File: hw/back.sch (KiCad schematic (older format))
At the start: 26 parts, among them J1 IDC_02X13, U1 OSRB38C9BA, U2 MCP1826S, U3 MCP1826S

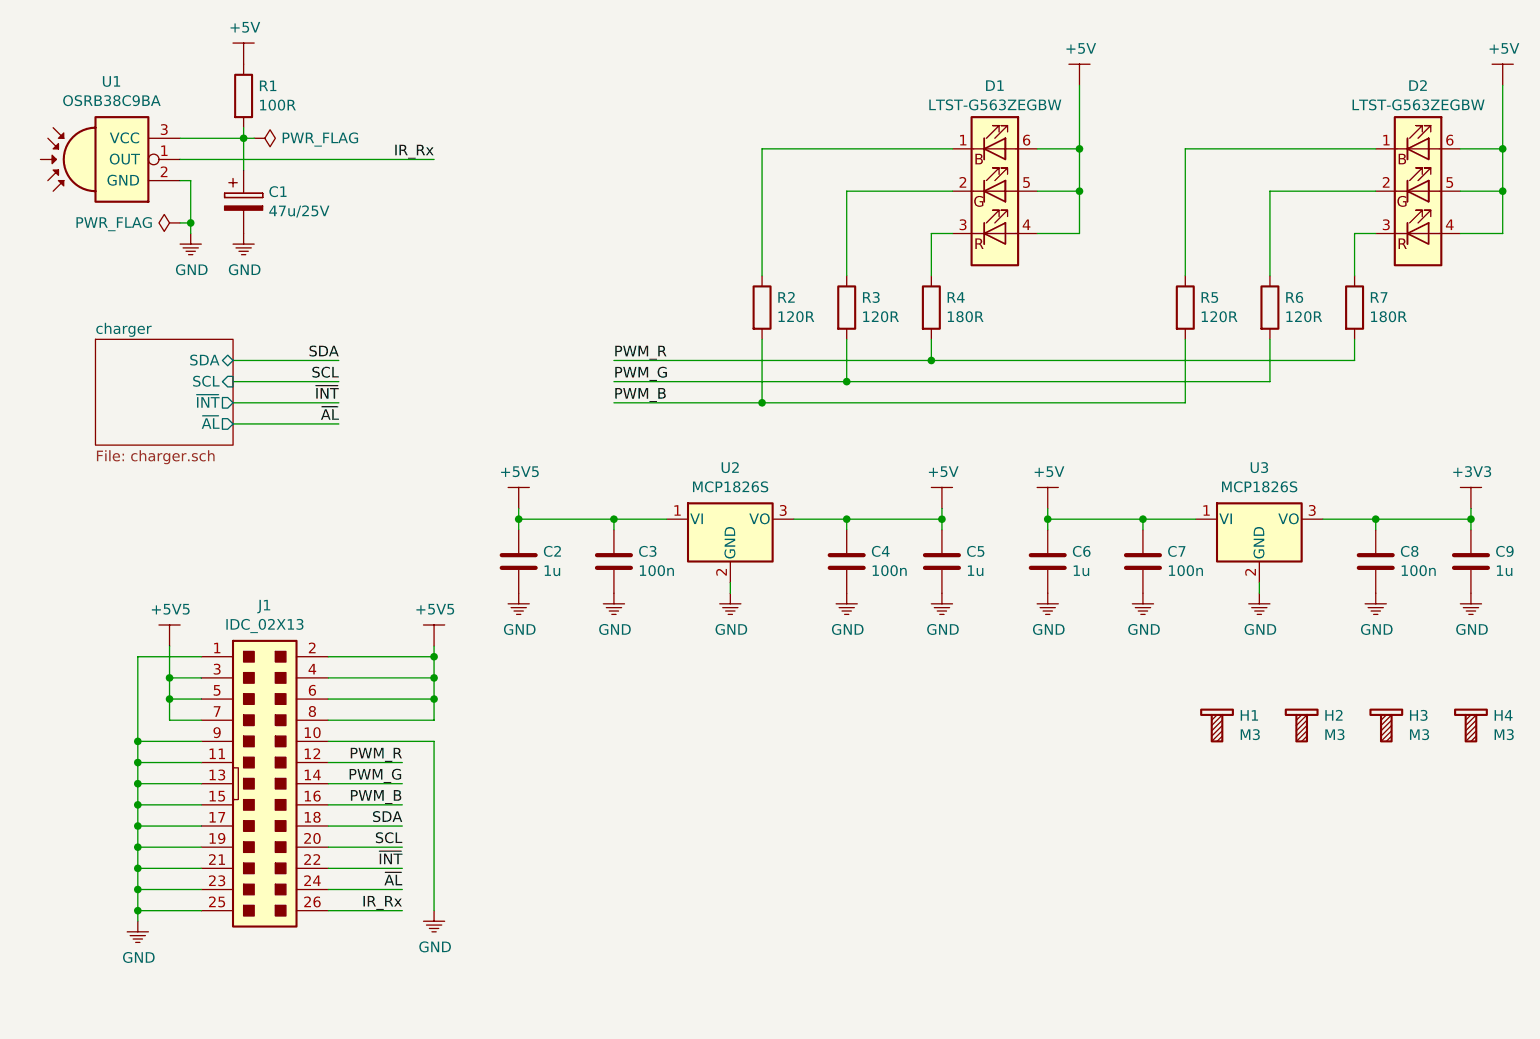
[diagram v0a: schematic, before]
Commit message: updated schematic
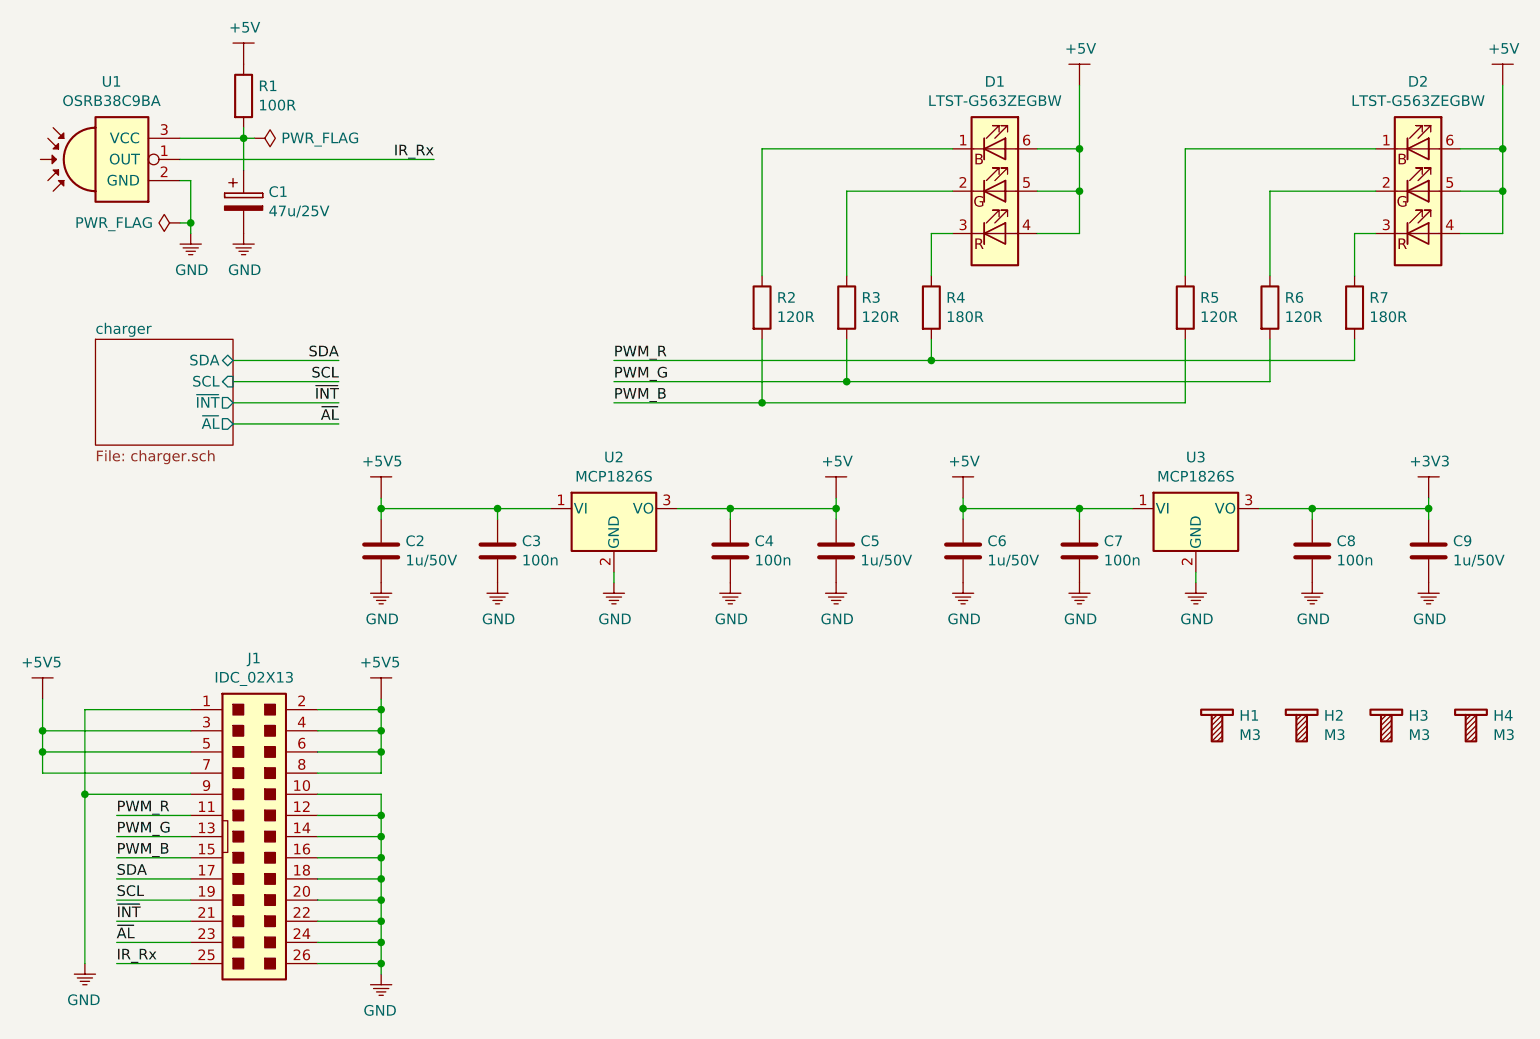
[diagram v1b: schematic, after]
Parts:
- C1: footprint (none) -> Capacitor_Tantalum_SMD:CP_EIA-7343-31_Kemet-D
- C2, C5, C6, C9: value 1u -> 1u/50V; footprint (none) -> Capacitor_SMD:C_0805_2012Metric
- C3, C4, C7, C8: footprint (none) -> Capacitor_SMD:C_0805_2012Metric
- D1, D2: footprint LEDs:LED_WS2812-PLCC6 -> KLIB_Opto:LED_RGB_5050-6
- J1: footprint Connectors:IDC_Header_Straight_26pins -> Connector_IDC:IDC-Header_2x13_P2.54mm_Vertical
- R1, R2, R3, R4, R5, R6, R7: footprint (none) -> Resistor_SMD:R_0805_2012Metric
- U1: footprint (none) -> KLIB_Opto:OSRB8C9BA_Horizontal
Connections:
- net GND: now also J1.12, J1.14, J1.16, J1.18, J1.20, J1.22, J1.24, J1.26; no longer J1.11, J1.13, J1.15, J1.17, J1.19, J1.21, J1.23, J1.25
- net IR_Rx: now also J1.25; no longer J1.26
- net PWM_B: now also J1.15; no longer J1.16
- net PWM_G: now also J1.13; no longer J1.14
- net PWM_R: now also J1.11; no longer J1.12
- net SCL: now also J1.19; no longer J1.20
- net SDA: now also J1.17; no longer J1.18
- net ~AL: now also J1.23; no longer J1.24
- net ~INT: now also J1.21; no longer J1.22
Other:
- moved on the sheet: C2, C3, C4, C5, C6, C7, C8, C9, J1, U2, U3
